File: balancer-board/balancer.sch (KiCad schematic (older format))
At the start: 23 parts, among them J1 Conn_01x08_Male, J2 Conn_01x17_Male, U1 74HCT164

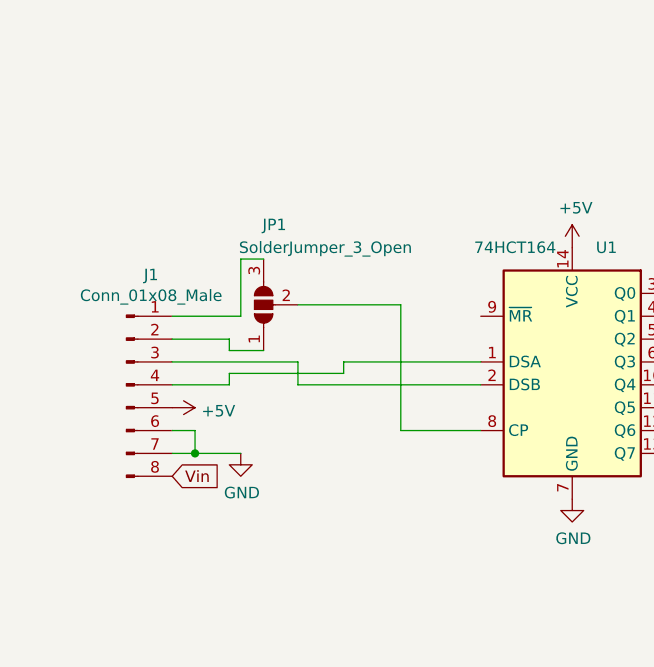
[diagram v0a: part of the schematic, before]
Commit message: multiple changes
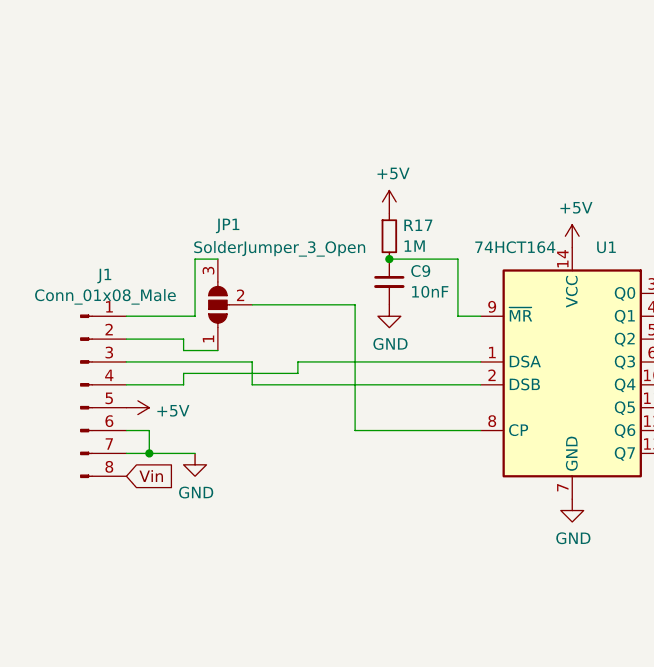
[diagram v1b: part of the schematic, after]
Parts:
- added C9: 10nF, Capacitor_SMD:C_0805_2012Metric_Pad1.15x1.40mm_HandSolder, symbol Device:C_Small
- added R17: 1M, Resistor_SMD:R_0805_2012Metric_Pad1.15x1.40mm_HandSolder, symbol Device:R_Small
- U1: footprint footprints:SOP-14 -> footprints:SO-14
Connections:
- net +5V: now also R17.1
- net GND: now also C9.2
- net at U1.9 (~MR): now also C9.1, R17.2
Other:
- moved on the sheet: J1, JP1
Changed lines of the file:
@@
 	10500 2600 9850 2600
 Wire Wire Line
-	2250 3300 2600 3300
-Wire Wire Line
-	1550 3400 1350 3400
+	1350 3400 1150 3400
 $Comp
 L power:GND #PWR0110
 U 1 1 5DA6FE6B
-P 1550 3400
-F 0 "#PWR0110" H 1550 3150 50  0001 C CNN
-F 1 "GND" H 1555 3227 50  0000 C CNN
-F 2 "" H 1550 3400 50  0001 C CNN
-F 3 "" H 1550 3400 50  0001 C CNN
-	1    1550 3400
-	1    0    0    -1
-$EndComp
-Text GLabel 1250 3500 2    50   Input ~ 0
+P 1350 3400
+F 0 "#PWR0110" H 1350 3150 50  0001 C CNN
+F 1 "GND" H 1355 3227 50  0000 C CNN
+F 2 "" H 1350 3400 50  0001 C CNN
+F 3 "" H 1350 3400 50  0001 C CNN
+	1    1350 3400
+	1    0    0    -1
+$EndComp
+Text GLabel 1050 3500 2    50   Input ~ 0
 Vin
 Wire Wire Line
-	1250 3100 1500 3100
-Wire Wire Line
-	1500 3100 1500 3050
-Wire Wire Line
-	1500 3050 2000 3050
-Wire Wire Line
-	2000 3050 2000 3000
-Wire Wire Line
-	2000 3000 2600 3000
-Wire Wire Line
-	1250 3000 1800 3000
-Wire Wire Line
-	1800 3000 1800 3100
-Wire Wire Line
-	1800 3100 2600 3100
+	1050 3100 1300 3100
+Wire Wire Line
+	1300 3100 1300 3050
+Wire Wire Line
+	1300 3050 1800 3050
+Wire Wire Line
+	1800 3050 1800 3000
+Wire Wire Line
+	1050 3000 1600 3000
+Wire Wire Line
+	1600 3000 1600 3100
 Text Notes 8900 6150 0    50   ~ 0
 TODO: HJT622 bypass / non-isolated 5V for the lowest TP4056
@@
 F 0 "U1" H 3150 3500 50  0000 C CNN
 F 1 "74HCT164" H 2750 3500 50  0000 C CNN
-F 2 "footprints:SOP-14" H 3900 2700 50  0001 C CNN
+F 2 "footprints:SO-14" H 3900 2700 50  0001 C CNN
 F 3 "https://assets.nexperia.com/documents/data-sheet/74HC_HCT164.pdf" H 3900 2700 50  0001 C CNN
 	1    3000 3000
@@
 L power:+5V #PWR0112
 U 1 1 5D908903
-P 1250 3200
-F 0 "#PWR0112" H 1250 3050 50  0001 C CNN
-F 1 "+5V" V 1265 3328 50  0000 L CNN
-F 2 "" H 1250 3200 50  0001 C CNN
-F 3 "" H 1250 3200 50  0001 C CNN
-	1    1250 3200
+P 1050 3200
+F 0 "#PWR0112" H 1050 3050 50  0001 C CNN
+F 1 "+5V" V 1065 3328 50  0000 L CNN
+F 2 "" H 1050 3200 50  0001 C CNN
+F 3 "" H 1050 3200 50  0001 C CNN
+	1    1050 3200
 	0    1    1    0
 $EndComp
@@
 	3400 5600 5400 5600
 Wire Wire Line
-	1500 2900 1500 2950
-Wire Wire Line
-	1250 2900 1500 2900
-Wire Wire Line
-	1550 2800 1550 2550
-Wire Wire Line
-	1250 2800 1550 2800
-Wire Wire Line
-	1500 2950 1650 2950
-Wire Wire Line
-	1550 2550 1650 2550
+	1300 2900 1300 2950
+Wire Wire Line
+	1050 2900 1300 2900
+Wire Wire Line
+	1350 2800 1350 2550
+Wire Wire Line
+	1050 2800 1350 2800
+Wire Wire Line
+	1300 2950 1450 2950
+Wire Wire Line
+	1350 2550 1450 2550
 $Comp
 L Jumper:SolderJumper_3_Open JP1
 U 1 1 5D94B181
-P 1650 2750
-F 0 "JP1" V 2000 2650 50  0000 L CNN
-F 1 "SolderJumper_3_Open" V 1900 2100 50  0000 L CNN
-F 2 "Jumper:SolderJumper-3_P1.3mm_Open_RoundedPad1.0x1.5mm" H 1650 2750 50  0001 C CNN
-F 3 "~" H 1650 2750 50  0001 C CNN
-	1    1650 2750
+P 1450 2750
+F 0 "JP1" V 1800 2650 50  0000 L CNN
+F 1 "SolderJumper_3_Open" V 1700 2100 50  0000 L CNN
+F 2 "Jumper:SolderJumper-3_P1.3mm_Open_RoundedPad1.0x1.5mm" H 1450 2750 50  0001 C CNN
+F 3 "~" H 1450 2750 50  0001 C CNN
+	1    1450 2750
 	0    -1   -1   0
 $EndComp
 Wire Wire Line
-	1800 2750 2250 2750
-Wire Wire Line
-	2250 2750 2250 3300
+	1600 2750 2050 2750
+Wire Wire Line
+	2050 2750 2050 3300
 $Comp
 L Connector:Conn_01x08_Male J1
 U 1 1 5D992C32
-P 1050 3100
-F 0 "J1" H 1158 3581 50  0000 C CNN
-F 1 "Conn_01x08_Male" H 1158 3490 50  0000 C CNN
-F 2 "Connector_PinHeader_2.54mm:PinHeader_1x08_P2.54mm_Vertical" H 1050 3100 50  0001 C CNN
-F 3 "~" H 1050 3100 50  0001 C CNN
-	1    1050 3100
-	1    0    0    -1
-$EndComp
-Wire Wire Line
-	1250 3300 1350 3300
-Wire Wire Line
-	1350 3300 1350 3400
-Connection ~ 1350 3400
-Wire Wire Line
-	1350 3400 1250 3400
+P 850 3100
+F 0 "J1" H 958 3581 50  0000 C CNN
+F 1 "Conn_01x08_Male" H 958 3490 50  0000 C CNN
+F 2 "Connector_PinHeader_2.54mm:PinHeader_1x08_P2.54mm_Vertical" H 850 3100 50  0001 C CNN
+F 3 "~" H 850 3100 50  0001 C CNN
+	1    850  3100
+	1    0    0    -1
+$EndComp
+Wire Wire Line
+	1050 3300 1150 3300
+Wire Wire Line
+	1150 3300 1150 3400
+Connection ~ 1150 3400
+Wire Wire Line
+	1150 3400 1050 3400
 $Comp
 L Jumper:SolderJumper_2_Open JP18
@@
 	1    0    0    -1
 $EndComp
+$Comp
+L Device:C_Small C9
+U 1 1 5DBC21DA
+P 2200 2650
+F 0 "C9" H 2292 2696 50  0000 L CNN
+F 1 "10nF" H 2292 2605 50  0000 L CNN
+F 2 "Capacitor_SMD:C_0805_2012Metric_Pad1.15x1.40mm_HandSolder" H 2200 2650 50  0001 C CNN
+F 3 "~" H 2200 2650 50  0001 C CNN
+	1    2200 2650
+	1    0    0    -1
+$EndComp
+Wire Wire Line
+	2050 3300 2600 3300
+$Comp
+L power:GND #PWR0114
+U 1 1 5DBF14DC
+P 2200 2750
+F 0 "#PWR0114" H 2200 2500 50  0001 C CNN
+F 1 "GND" H 2205 2577 50  0000 C CNN
+F 2 "" H 2200 2750 50  0001 C CNN
+F 3 "" H 2200 2750 50  0001 C CNN
+	1    2200 2750
+	1    0    0    -1
+$EndComp
+Wire Wire Line
+	2600 2800 2500 2800
+$Comp
+L Device:R_Small R17
+U 1 1 5DC0CEAE
+P 2200 2450
+F 0 "R17" H 2259 2496 50  0000 L CNN
+F 1 "1M" H 2259 2405 50  0000 L CNN
+F 2 "Resistor_SMD:R_0805_2012Metric_Pad1.15x1.40mm_HandSolder" H 2200 2450 50  0001 C CNN
+F 3 "~" H 2200 2450 50  0001 C CNN
+	1    2200 2450
+	1    0    0    -1
+$EndComp
+Connection ~ 2200 2550
+$Comp
+L power:+5V #PWR0115
+U 1 1 5DC0D520
+P 2200 2350
+F 0 "#PWR0115" H 2200 2200 50  0001 C CNN
+F 1 "+5V" H 2215 2523 50  0000 C CNN
+F 2 "" H 2200 2350 50  0001 C CNN
+F 3 "" H 2200 2350 50  0001 C CNN
+	1    2200 2350
+	1    0    0    -1
+$EndComp
+Wire Wire Line
+	2500 2800 2500 2550
+Wire Wire Line
+	2200 2550 2500 2550
+Wire Wire Line
+	1800 3000 2600 3000
+Wire Wire Line
+	1600 3100 2600 3100
 $EndSCHEMATC
